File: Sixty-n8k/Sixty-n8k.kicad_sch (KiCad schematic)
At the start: 67 parts, among them J1 USB4085-GF-A_REVB, J2 SD_CARD_PORT, J3 Conn_02x32_Odd_Even, J4 Conn_01x02, SW1 RESET, SW2 DEBUG, U1 74LS05, U10 74HC164, U11 74LS393, U12 22V10C, U13 74LS148, U14 MC68901P, U16 74LS138, U17 CH340C, U19 74LS21, U2 NE555P, U3 AM29F040-70, U4 AS6C4008, U6 68000D, U7 AS6C4008, U8 AM29F040-70, U9 TPD4E1U06DBVR, X1 7.3728Mhz

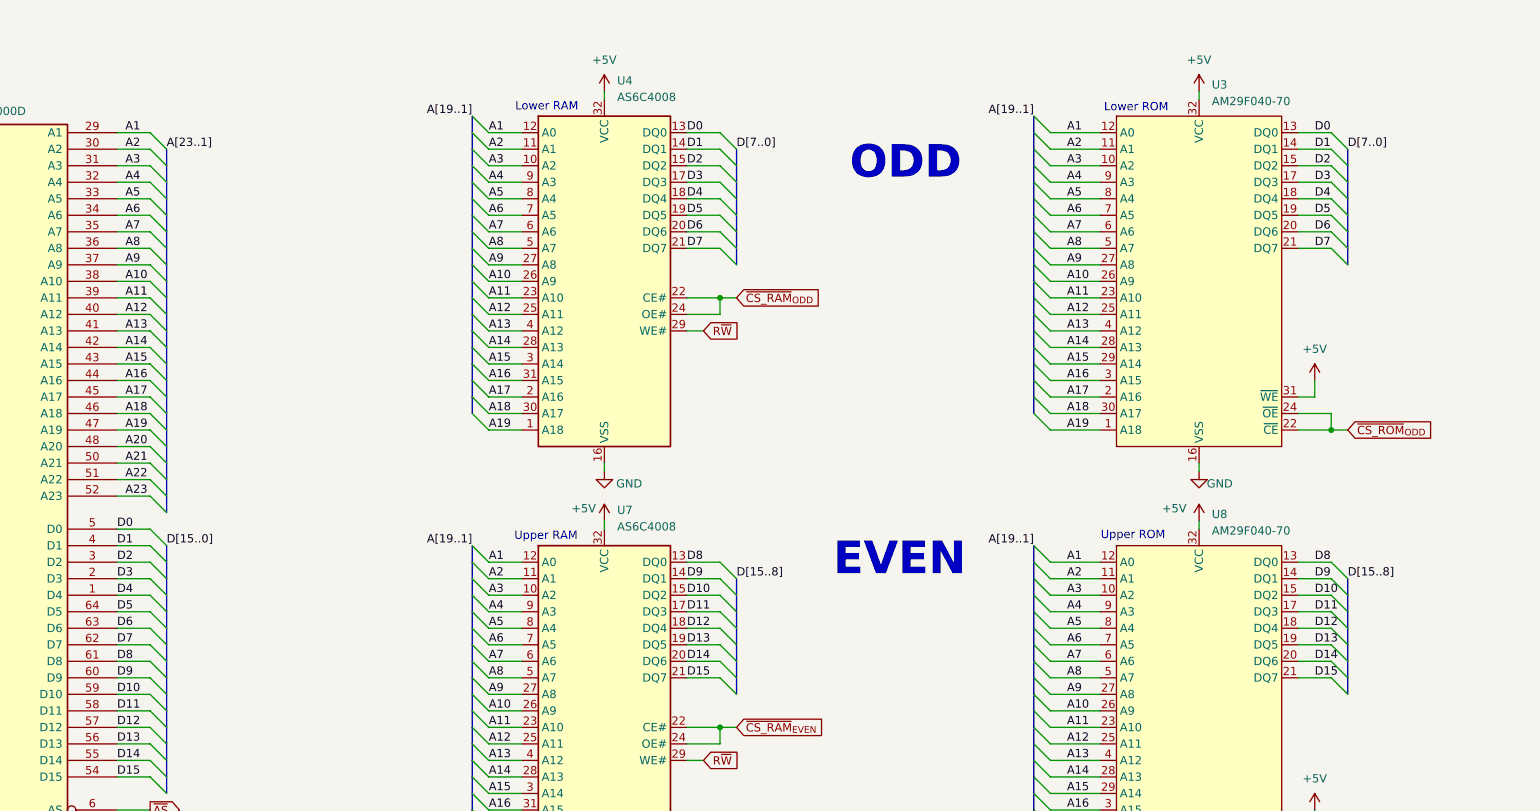
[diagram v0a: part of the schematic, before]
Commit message: Formatting changes
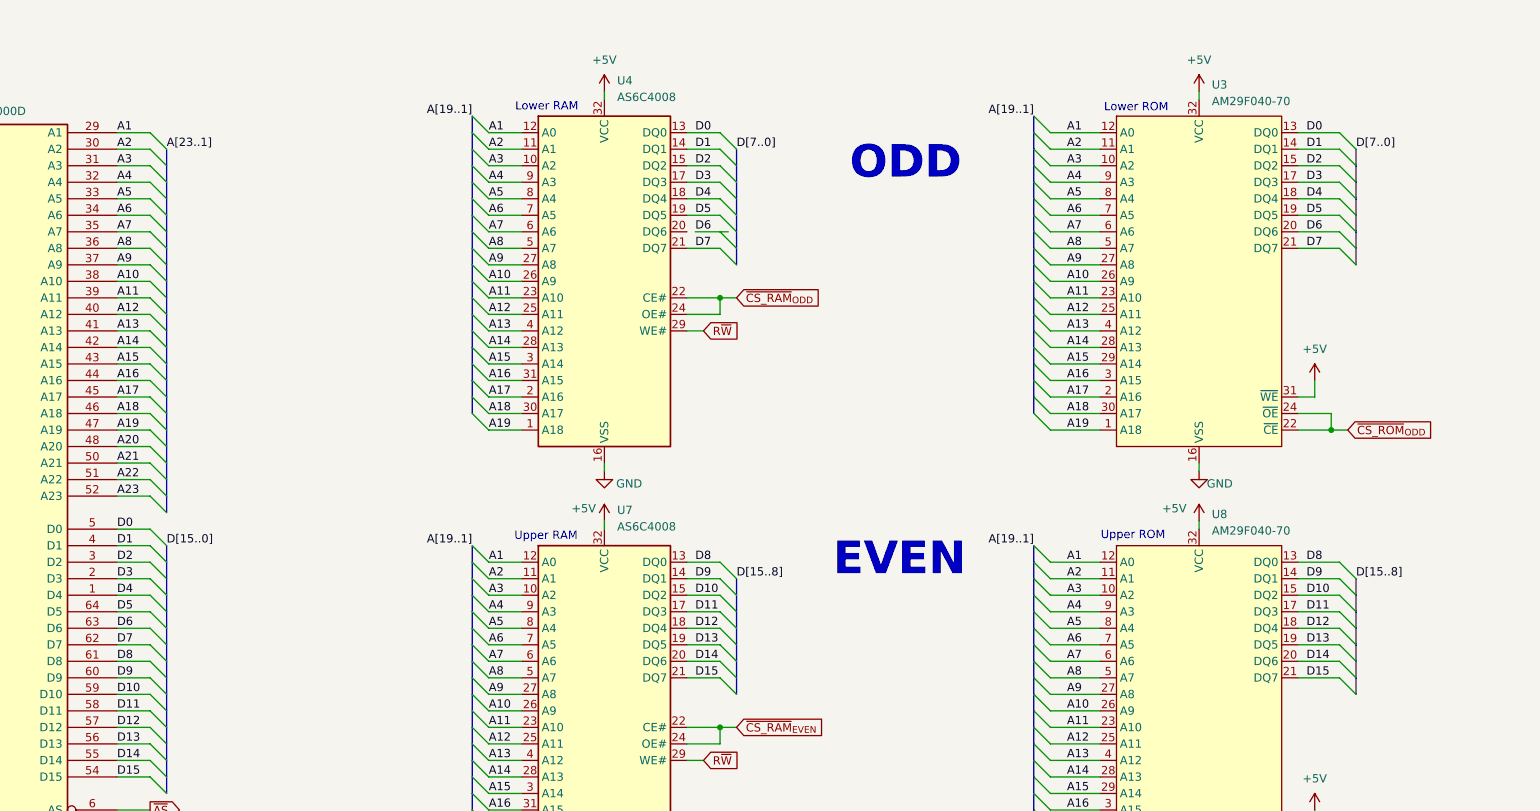
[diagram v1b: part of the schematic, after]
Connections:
- net D6: no longer U4.20 (DQ6)

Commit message: Removed pullup on RWb
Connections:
- net D6: now also U4.20 (DQ6)
- net R~{W}: no longer RN3.5 (R4)
- net ~{BERR}: now also J3.40 (Pin_40); no longer J3.44 (Pin_44)
- net ~{BGACK}: now also J3.46 (Pin_46); no longer J3.60 (Pin_60)
- net ~{BG}: now also J3.42 (Pin_42); no longer J3.40 (Pin_40)
- net ~{BR}: now also J3.44 (Pin_44); no longer J3.42 (Pin_42)
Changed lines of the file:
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@@
   (no_connect (at 62.23 152.4))
   (no_connect (at 361.95 194.31))
-  (no_connect (at 58.42 327.66))
   (no_connect (at 527.05 199.39))
   (no_connect (at 336.55 327.66))
@@
   (no_connect (at 273.05 278.13))
   (no_connect (at 361.95 196.85))
+  (no_connect (at 532.13 90.17))
   (no_connect (at 438.15 294.64))
   (no_connect (at 194.31 208.28))
@@
     (stroke (width 0) (type default))
   )
-  (wire (pts (xy 529.59 90.17) (xy 532.13 90.17))
-    (stroke (width 0) (type default))
-  )
   (wire (pts (xy 323.85 48.26) (xy 328.93 48.26))
     (stroke (width 0) (type default))
@@
     (stroke (width 0) (type default))
   )
-  (wire (pts (xy 355.6 50.8) (xy 359.41 50.8))
+  (wire (pts (xy 354.33 50.8) (xy 359.41 50.8))
     (stroke (width 0) (type default))
   )
@@
     (stroke (width 0) (type default))
   )
-  (wire (pts (xy 58.42 320.04) (xy 60.96 320.04))
+  (wire (pts (xy 58.42 322.58) (xy 60.96 322.58))
     (stroke (width 0) (type default))
   )
@@
     (stroke (width 0) (type default))
   )
-  (wire (pts (xy 359.41 50.8) (xy 360.68 50.8))
-    (stroke (width 0) (type default))
-  )
   (wire (pts (xy 323.85 134.62) (xy 328.93 134.62))
     (stroke (width 0) (type default))
@@
     (stroke (width 0) (type solid))
   )
-  (wire (pts (xy 58.42 322.58) (xy 60.96 322.58))
+  (wire (pts (xy 58.42 325.12) (xy 60.96 325.12))
     (stroke (width 0) (type default))
   )
@@
     (stroke (width 0) (type default))
   )
-  (wire (pts (xy 58.42 345.44) (xy 60.96 345.44))
+  (wire (pts (xy 58.42 327.66) (xy 60.96 327.66))
     (stroke (width 0) (type default))
   )
@@
     (stroke (width 0) (type default))
   )
-  (wire (pts (xy 58.42 325.12) (xy 60.96 325.12))
+  (wire (pts (xy 58.42 320.04) (xy 60.96 320.04))
     (stroke (width 0) (type default))
   )
@@
     )
   )
-  (global_label "~{BR}" (shape output) (at 60.96 322.58 0) (fields_autoplaced)
+  (global_label "~{BR}" (shape output) (at 60.96 325.12 0) (fields_autoplaced)
     (effects (font (size 1.27 1.27)) (justify left))
-    (property "Intersheetrefs" "${INTERSHEET_REFS}" (at 66.4058 322.58 0)
+    (property "Intersheetrefs" "${INTERSHEET_REFS}" (at 66.4058 325.12 0)
       (effects (font (size 1.27 1.27)) (justify left) hide)
     )
@@
     )
   )
-  (global_label "R~{W}" (shape input) (at 529.59 90.17 180) (fields_autoplaced)
-    (effects (font (size 1.27 1.27)) (justify right))
-    (property "Intersheetrefs" "${INTERSHEET_REFS}" (at 523.9628 90.17 0)
-      (effects (font (size 1.27 1.27)) (justify right) hide)
-    )
-  )
   (global_label "~{LDS}" (shape input) (at 231.14 222.25 180) (fields_autoplaced)
     (effects (font (size 1.27 1.27)) (justify right))
@@
     )
   )
-  (global_label "~{BERR}" (shape input) (at 60.96 325.12 0) (fields_autoplaced)
+  (global_label "~{BERR}" (shape input) (at 60.96 320.04 0) (fields_autoplaced)
     (effects (font (size 1.27 1.27)) (justify left))
-    (property "Intersheetrefs" "${INTERSHEET_REFS}" (at 68.8248 325.12 0)
+    (property "Intersheetrefs" "${INTERSHEET_REFS}" (at 68.8248 320.04 0)
       (effects (font (size 1.27 1.27)) (justify left) hide)
     )
@@
     )
   )
-  (global_label "~{BG}" (shape input) (at 60.96 320.04 0) (fields_autoplaced)
+  (global_label "~{BG}" (shape input) (at 60.96 322.58 0) (fields_autoplaced)
     (effects (font (size 1.27 1.27)) (justify left))
-    (property "Intersheetrefs" "${INTERSHEET_REFS}" (at 66.4058 320.04 0)
+    (property "Intersheetrefs" "${INTERSHEET_REFS}" (at 66.4058 322.58 0)
       (effects (font (size 1.27 1.27)) (justify left) hide)
     )
@@
     )
   )
-  (global_label "~{BGACK}" (shape output) (at 60.96 345.44 0) (fields_autoplaced)
+  (global_label "~{BGACK}" (shape output) (at 60.96 327.66 0) (fields_autoplaced)
     (effects (font (size 1.27 1.27)) (justify left))
-    (property "Intersheetrefs" "${INTERSHEET_REFS}" (at 70.0344 345.44 0)
+    (property "Intersheetrefs" "${INTERSHEET_REFS}" (at 70.0344 327.66 0)
       (effects (font (size 1.27 1.27)) (justify left) hide)
     )
